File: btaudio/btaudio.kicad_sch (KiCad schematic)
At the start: 51 parts, among them J1 BAT_CON, J2 USB_C_Receptacle_USB2.0_16P, J3 Audio, SW1 POWER_SW, SW2 PLAY/VOL+, SW3 PAUSE/VOL-, SW4 PREV/BT PAIRING, SW6 SOFT RESET, U1 EWM104-BT5125, U2 PCM5102AQPWRQ1, U3 TPA6132A2RTET, U5 MCP1700x-330xxTT

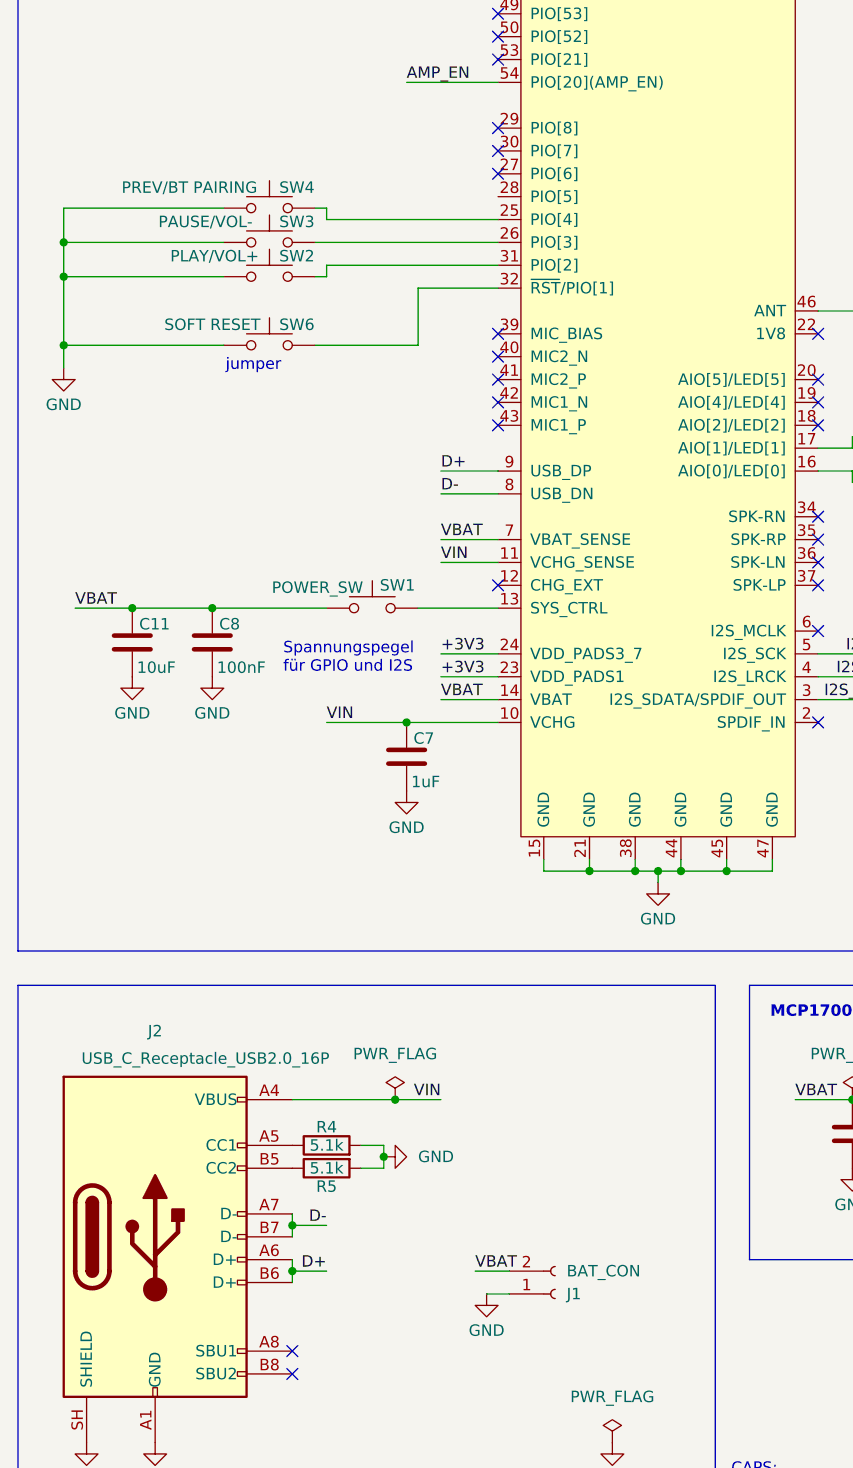
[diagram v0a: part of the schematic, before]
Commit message: primary layout done
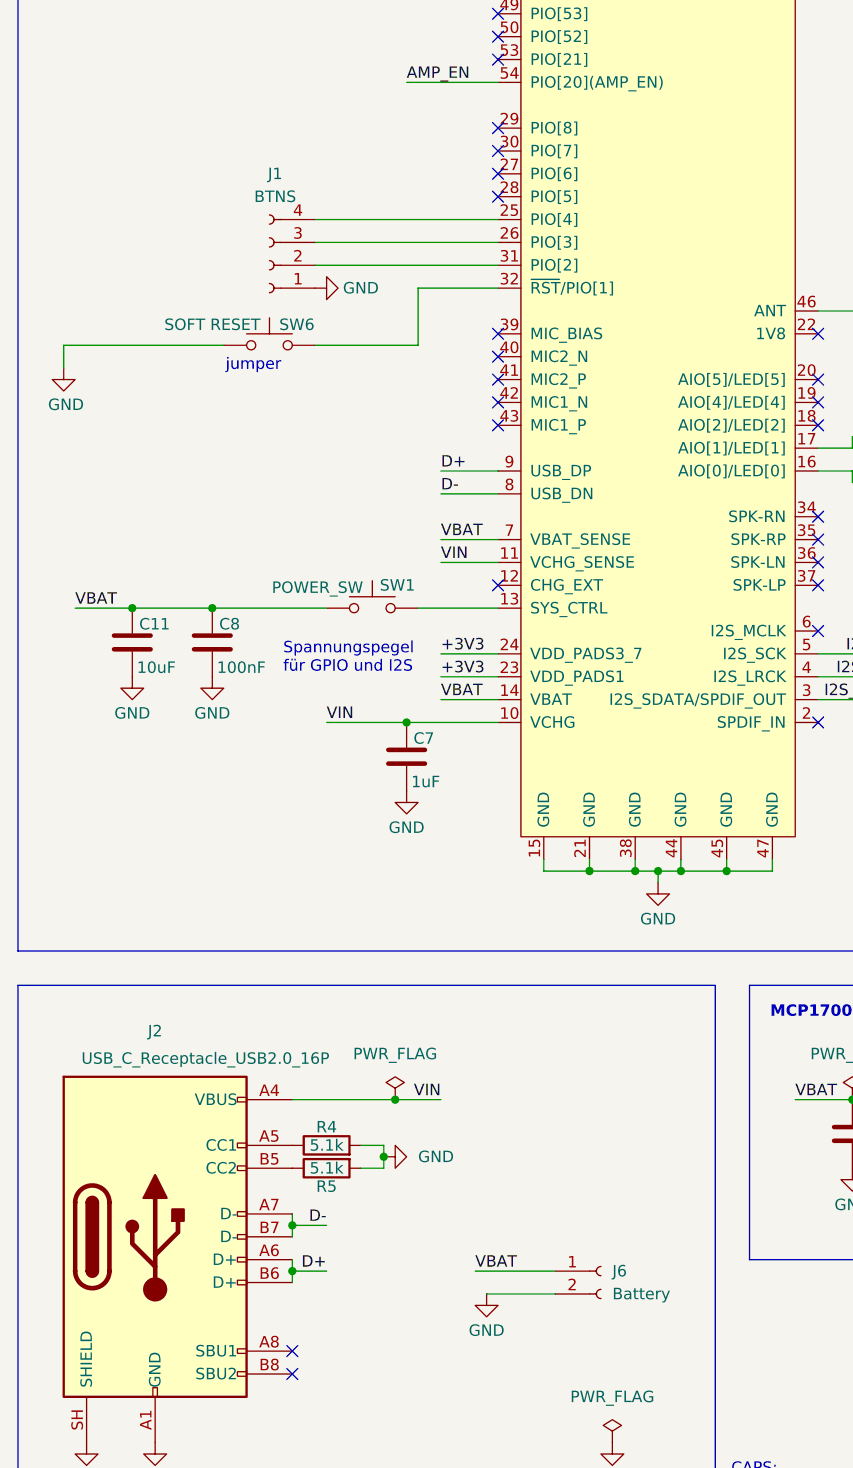
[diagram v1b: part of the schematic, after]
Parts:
- removed J1: BAT_CON, Connector_JST:JST_SH_SM02B-SRSS-TB_1x02-1MP_P1.00mm_Horizontal, symbol Connector:Conn_01x02_Socket
- removed SW2: PLAY/VOL+, Button_Switch_SMD:SW_SPST_TS-1088-xR020, symbol Switch:SW_Push
- removed SW3: PAUSE/VOL-, Button_Switch_SMD:SW_SPST_TS-1088-xR020, symbol Switch:SW_Push
- removed SW4: PREV/BT PAIRING, Button_Switch_SMD:SW_SPST_TS-1088-xR020, symbol Switch:SW_Push
- added J1: BTNS, Connector_PinHeader_2.54mm:PinHeader_1x04_P2.54mm_Vertical, symbol Connector:Conn_01x04_Socket
- added J6: Battery, Connector_PinHeader_2.54mm:PinHeader_1x02_P2.54mm_Vertical, symbol Connector:Conn_01x02_Socket
- J3: footprint PCM_Crystal_Handsoldering_AKL:Resonator_SMD-3Pin_7.2x3.0mm_BigPads -> Aux-Pads:aux-pads
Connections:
- net GND: now also J1.1 (Pin_1), J6.2 (Pin_2)
- net VBAT: now also J6.1 (Pin_1)
- net at U1.26 (PIO[3]): now also J1.3 (Pin_3)
- net at U1.31 (PIO[2]): now also J1.2 (Pin_2)
- net at U1.25 (PIO[4]): now also J1.4 (Pin_4)
- no-connect marks 27 -> 28
